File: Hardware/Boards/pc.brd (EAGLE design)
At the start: 17.4 x 31.7 mm, 4 parts

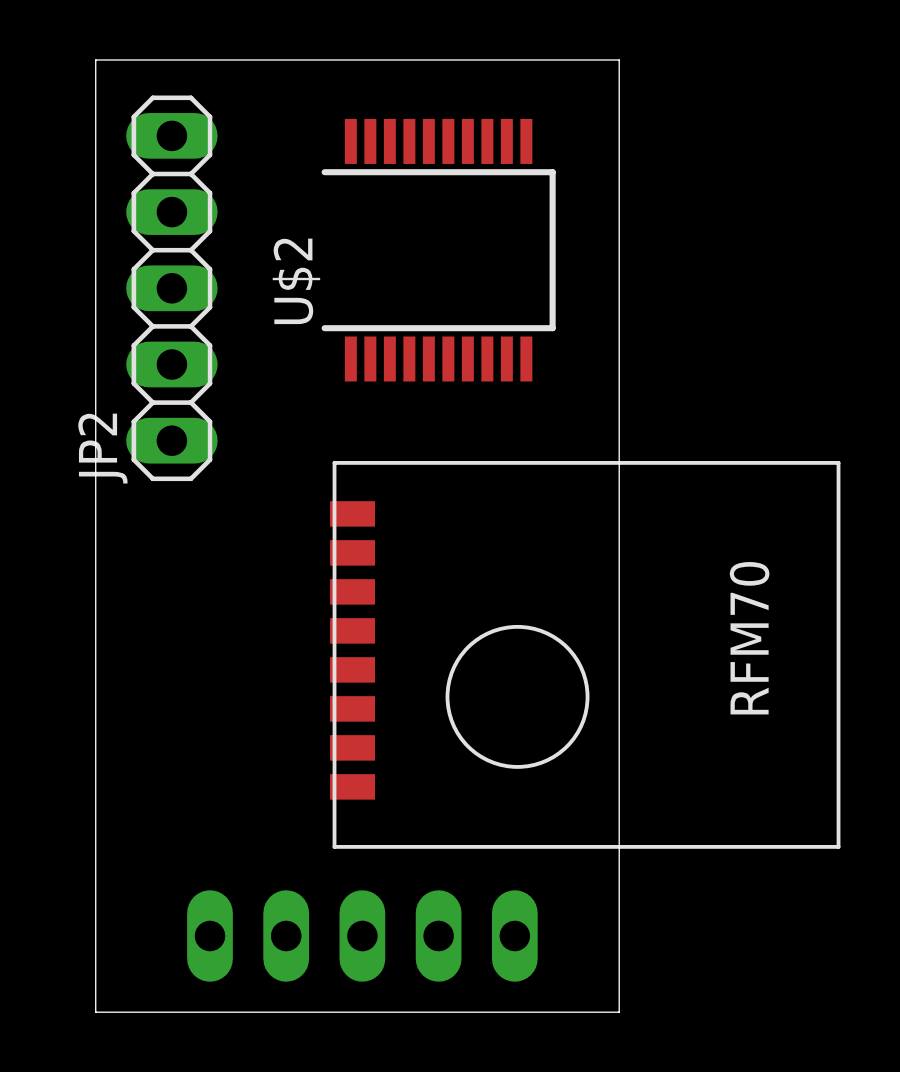
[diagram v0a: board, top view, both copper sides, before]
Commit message: a
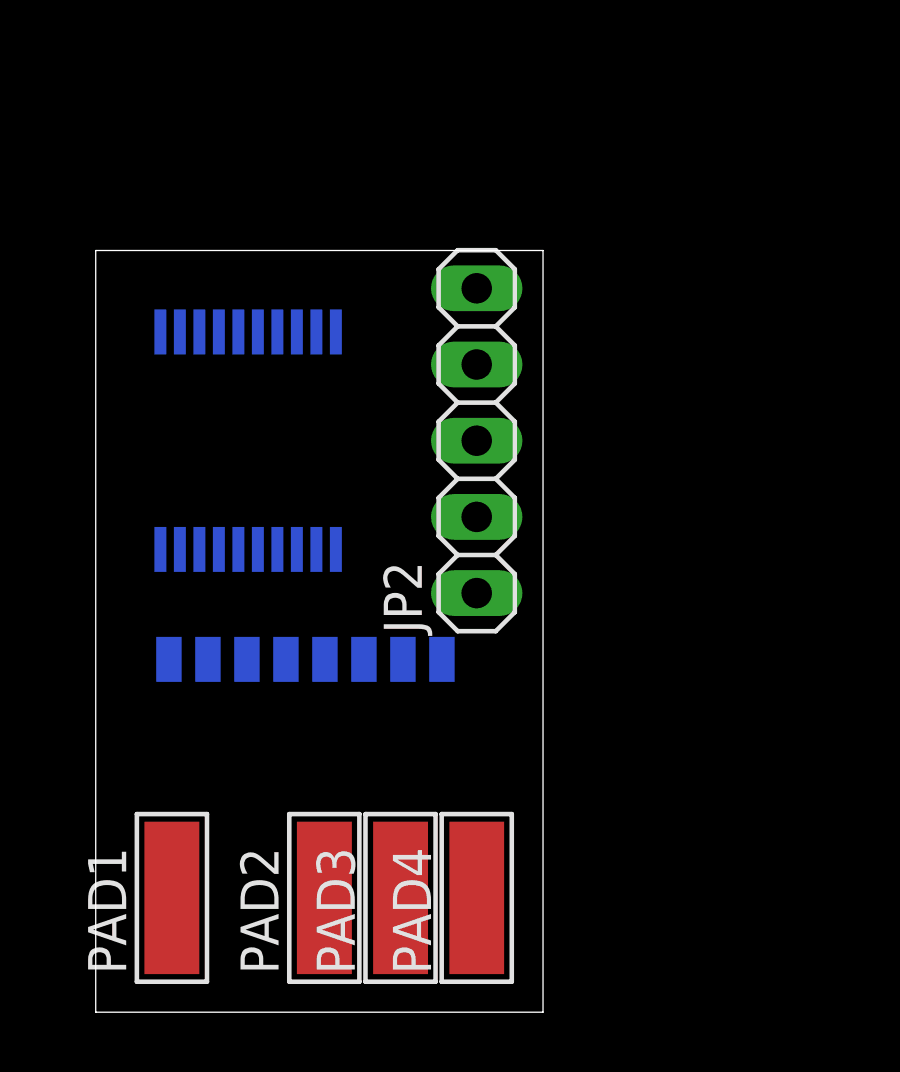
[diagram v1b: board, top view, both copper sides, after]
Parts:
- removed JP3: (no value), pinhead:1X05/90
- added PAD1, PAD2, PAD3, PAD4: WIREPADSMD5-1,8, wirepad:5-1,8
- moved U$1 27.9 mm to (2.54, -2.54), flipped to the bottom, turned to 180 degrees
- moved JP2 11.4 mm to (12.7, 19.1)
- moved U$2 8.98 mm to (5.08, 19.1), flipped to the bottom
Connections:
- net N$17: now also PAD1.1; no longer JP3.1
- net N$33: now also PAD3.1; no longer JP3.4
- net N$34: now also PAD2.1; no longer JP3.3
- net N$5: now also PAD4.1; no longer JP3.5
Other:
- board size 17.4 x 31.7 mm -> 14.9 x 25.4 mm
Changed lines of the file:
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@@
 <setting verticaltext="up"/>
 </settings>
-<grid distance="0.05" unitdist="inch" unit="inch" style="lines" multiple="1" display="no" altdistance="0.025" altunitdist="inch" altunit="inch"/>
+<grid distance="0.05" unitdist="inch" unit="mm" style="lines" multiple="1" display="no" altdistance="0.025" altunitdist="inch" altunit="inch"/>
 <layers>
 <layer number="1" name="Top" color="4" fill="1" visible="yes" active="yes"/>
@@
 <board>
 <plain>
-<wire x1="0" y1="0" x2="17.45" y2="0" width="0" layer="20"/>
-<wire x1="17.45" y1="0" x2="17.45" y2="31.74" width="0" layer="20"/>
-<wire x1="17.45" y1="31.74" x2="0" y2="31.74" width="0" layer="20"/>
-<wire x1="0" y1="31.74" x2="0" y2="0" width="0" layer="20"/>
+<wire x1="0" y1="0" x2="14.91" y2="0" width="0" layer="20"/>
+<wire x1="14.91" y1="0" x2="14.91" y2="25.39" width="0" layer="20"/>
+<wire x1="14.91" y1="25.39" x2="0" y2="25.39" width="0" layer="20"/>
+<wire x1="0" y1="25.39" x2="0" y2="0" width="0" layer="20"/>
 </plain>
 <attributes>
@@
 </autorouter>
 <elements>
-<element name="U$1" library="rfm70" package="RFM70" value="RFM70" x="22.86" y="16.51" rot="R270"/>
-<element name="U$2" library="microchip" package="SSOP20" value="PIC16F690" x="11.43" y="25.4"/>
-<element name="JP2" library="pinhead" package="1X05" value="Prog" x="2.54" y="24.13" rot="R90"/>
-<element name="JP3" library="pinhead" package="1X05/90" value="" x="8.89" y="6.35" rot="MR0"/>
+<element name="U$1" library="rfm70" package="RFM70" value="RFM70" x="2.54" y="-2.54" rot="MR180"/>
+<element name="U$2" library="microchip" package="SSOP20" value="PIC16F690" x="5.08" y="19.05" rot="MR0"/>
+<element name="JP2" library="pinhead" package="1X05" value="Prog" x="12.7" y="19.05" rot="R90"/>
+<element name="PAD1" library="wirepad" package="5-1,8" value="WIREPADSMD5-1,8" x="2.54" y="3.81"/>
+<element name="PAD2" library="wirepad" package="5-1,8" value="WIREPADSMD5-1,8" x="7.62" y="3.81"/>
+<element name="PAD3" library="wirepad" package="5-1,8" value="WIREPADSMD5-1,8" x="10.16" y="3.81"/>
+<element name="PAD4" library="wirepad" package="5-1,8" value="WIREPADSMD5-1,8" x="12.7" y="3.81"/>
 </elements>
 <signals>
@@
 <contactref element="U$1" pad="GND"/>
 <contactref element="JP2" pad="3"/>
-<contactref element="JP3" pad="5"/>
-<wire x1="3.81" y1="2.54" x2="8.56" y2="16.61" width="0" layer="19" extent="1-1"/>
-<wire x1="8.505" y1="29.025" x2="3.81" y2="2.54" width="0" layer="19" extent="1-1"/>
-<wire x1="2.54" y1="24.13" x2="8.505" y2="29.025" width="0" layer="19" extent="1-1"/>
+<contactref element="PAD4" pad="1"/>
+<wire x1="8.005" y1="22.675" x2="12.7" y2="19.05" width="0" layer="19" extent="1-1"/>
+<wire x1="2.44" y1="11.76" x2="8.005" y2="22.675" width="0" layer="19" extent="1-1"/>
+<wire x1="12.7" y1="3.81" x2="2.44" y2="11.76" width="0" layer="19" extent="1-1"/>
 </signal>
 <signal name="N$12">
 <contactref element="U$1" pad="MISO"/>
 <contactref element="U$2" pad="13"/>
-<wire x1="8.56" y1="8.81" x2="13.055" y2="29.025" width="0" layer="19" extent="1-1"/>
+<wire x1="10.24" y1="11.76" x2="3.455" y2="22.675" width="0" layer="19" extent="1-1"/>
 </signal>
 <signal name="N$17">
@@
 <contactref element="U$1" pad="VDD"/>
 <contactref element="JP2" pad="2"/>
-<contactref element="JP3" pad="1"/>
-<wire x1="13.97" y1="2.54" x2="8.56" y2="15.31" width="0" layer="19" extent="1-1"/>
-<wire x1="8.505" y1="21.775" x2="13.97" y2="2.54" width="0" layer="19" extent="1-1"/>
-<wire x1="2.54" y1="21.59" x2="8.505" y2="21.775" width="0" layer="19" extent="1-1"/>
+<contactref element="PAD1" pad="1"/>
+<wire x1="8.005" y1="15.425" x2="12.7" y2="16.51" width="0" layer="19" extent="1-1"/>
+<wire x1="3.74" y1="11.76" x2="8.005" y2="15.425" width="0" layer="19" extent="1-1"/>
+<wire x1="2.54" y1="3.81" x2="8.005" y2="15.425" width="0" layer="19" extent="1-1"/>
 </signal>
 <signal name="N$18">
 <contactref element="U$2" pad="19"/>
 <contactref element="JP2" pad="4"/>
-<wire x1="2.54" y1="26.67" x2="9.155" y2="29.025" width="0" layer="19" extent="1-1"/>
+<wire x1="12.7" y1="21.59" x2="7.355" y2="22.675" width="0" layer="19" extent="1-1"/>
 </signal>
 <signal name="N$19">
 <contactref element="U$2" pad="18"/>
 <contactref element="JP2" pad="5"/>
-<wire x1="2.54" y1="29.21" x2="9.805" y2="29.025" width="0" layer="19" extent="1-1"/>
+<wire x1="12.7" y1="24.13" x2="6.705" y2="22.675" width="0" layer="19" extent="1-1"/>
 </signal>
 <signal name="N$16">
 <contactref element="U$2" pad="17"/>
 <contactref element="U$1" pad="CE"/>
-<wire x1="8.56" y1="14.01" x2="10.455" y2="29.025" width="0" layer="19" extent="1-1"/>
+<wire x1="5.04" y1="11.76" x2="6.055" y2="22.675" width="0" layer="19" extent="1-1"/>
 </signal>
 <signal name="N$20">
 <contactref element="U$2" pad="16"/>
 <contactref element="U$1" pad="CSN"/>
-<wire x1="8.56" y1="12.71" x2="11.105" y2="29.025" width="0" layer="19" extent="1-1"/>
+<wire x1="6.34" y1="11.76" x2="5.405" y2="22.675" width="0" layer="19" extent="1-1"/>
 </signal>
 <signal name="N$21">
 <contactref element="U$2" pad="14"/>
 <contactref element="U$1" pad="IRQ"/>
-<wire x1="8.56" y1="7.51" x2="12.405" y2="29.025" width="0" layer="19" extent="1-1"/>
+<wire x1="11.54" y1="11.76" x2="4.105" y2="22.675" width="0" layer="19" extent="1-1"/>
 </signal>
 <signal name="N$22">
 <contactref element="U$2" pad="11"/>
 <contactref element="U$1" pad="SCK"/>
-<wire x1="8.56" y1="11.41" x2="14.355" y2="29.025" width="0" layer="19" extent="1-1"/>
+<wire x1="7.64" y1="11.76" x2="2.155" y2="22.675" width="0" layer="19" extent="1-1"/>
 </signal>
 <signal name="N$23">
 <contactref element="U$2" pad="9"/>
 <contactref element="U$1" pad="MOSI"/>
-<wire x1="8.56" y1="10.11" x2="13.705" y2="21.775" width="0" layer="19" extent="1-1"/>
+<wire x1="8.94" y1="11.76" x2="2.805" y2="15.425" width="0" layer="19" extent="1-1"/>
 </signal>
 <signal name="N$25">
 <contactref element="U$2" pad="4"/>
 <contactref element="JP2" pad="1"/>
-<wire x1="2.54" y1="19.05" x2="10.455" y2="21.775" width="0" layer="19" extent="1-1"/>
+<wire x1="12.7" y1="13.97" x2="6.055" y2="15.425" width="0" layer="19" extent="1-1"/>
 </signal>
 <signal name="N$28">
@@
 <signal name="N$33">
 <contactref element="U$2" pad="10"/>
-<contactref element="JP3" pad="4"/>
-<wire x1="6.35" y1="2.54" x2="14.355" y2="21.775" width="0" layer="19" extent="1-1"/>
+<contactref element="PAD3" pad="1"/>
+<wire x1="10.16" y1="3.81" x2="2.155" y2="15.425" width="0" layer="19" extent="1-1"/>
 </signal>
 <signal name="N$34">
 <contactref element="U$2" pad="12"/>
-<contactref element="JP3" pad="3"/>
-<wire x1="8.89" y1="2.54" x2="13.705" y2="29.025" width="0" layer="19" extent="1-1"/>
+<contactref element="PAD2" pad="1"/>
+<wire x1="7.62" y1="3.81" x2="2.805" y2="22.675" width="0" layer="19" extent="1-1"/>
 </signal>
 </signals>
